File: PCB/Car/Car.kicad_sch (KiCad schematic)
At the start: 16 parts, among them J1 L1, J10 FL2, J11 FLT, J2 L2, J3 R1, J4 R2, J5 R1+2, J6 L1+2, J7 Conn_01x03, J8 pi zero 2 w, J9 FL1, U3 YAAJ_DCDC_StepDown_LM2596

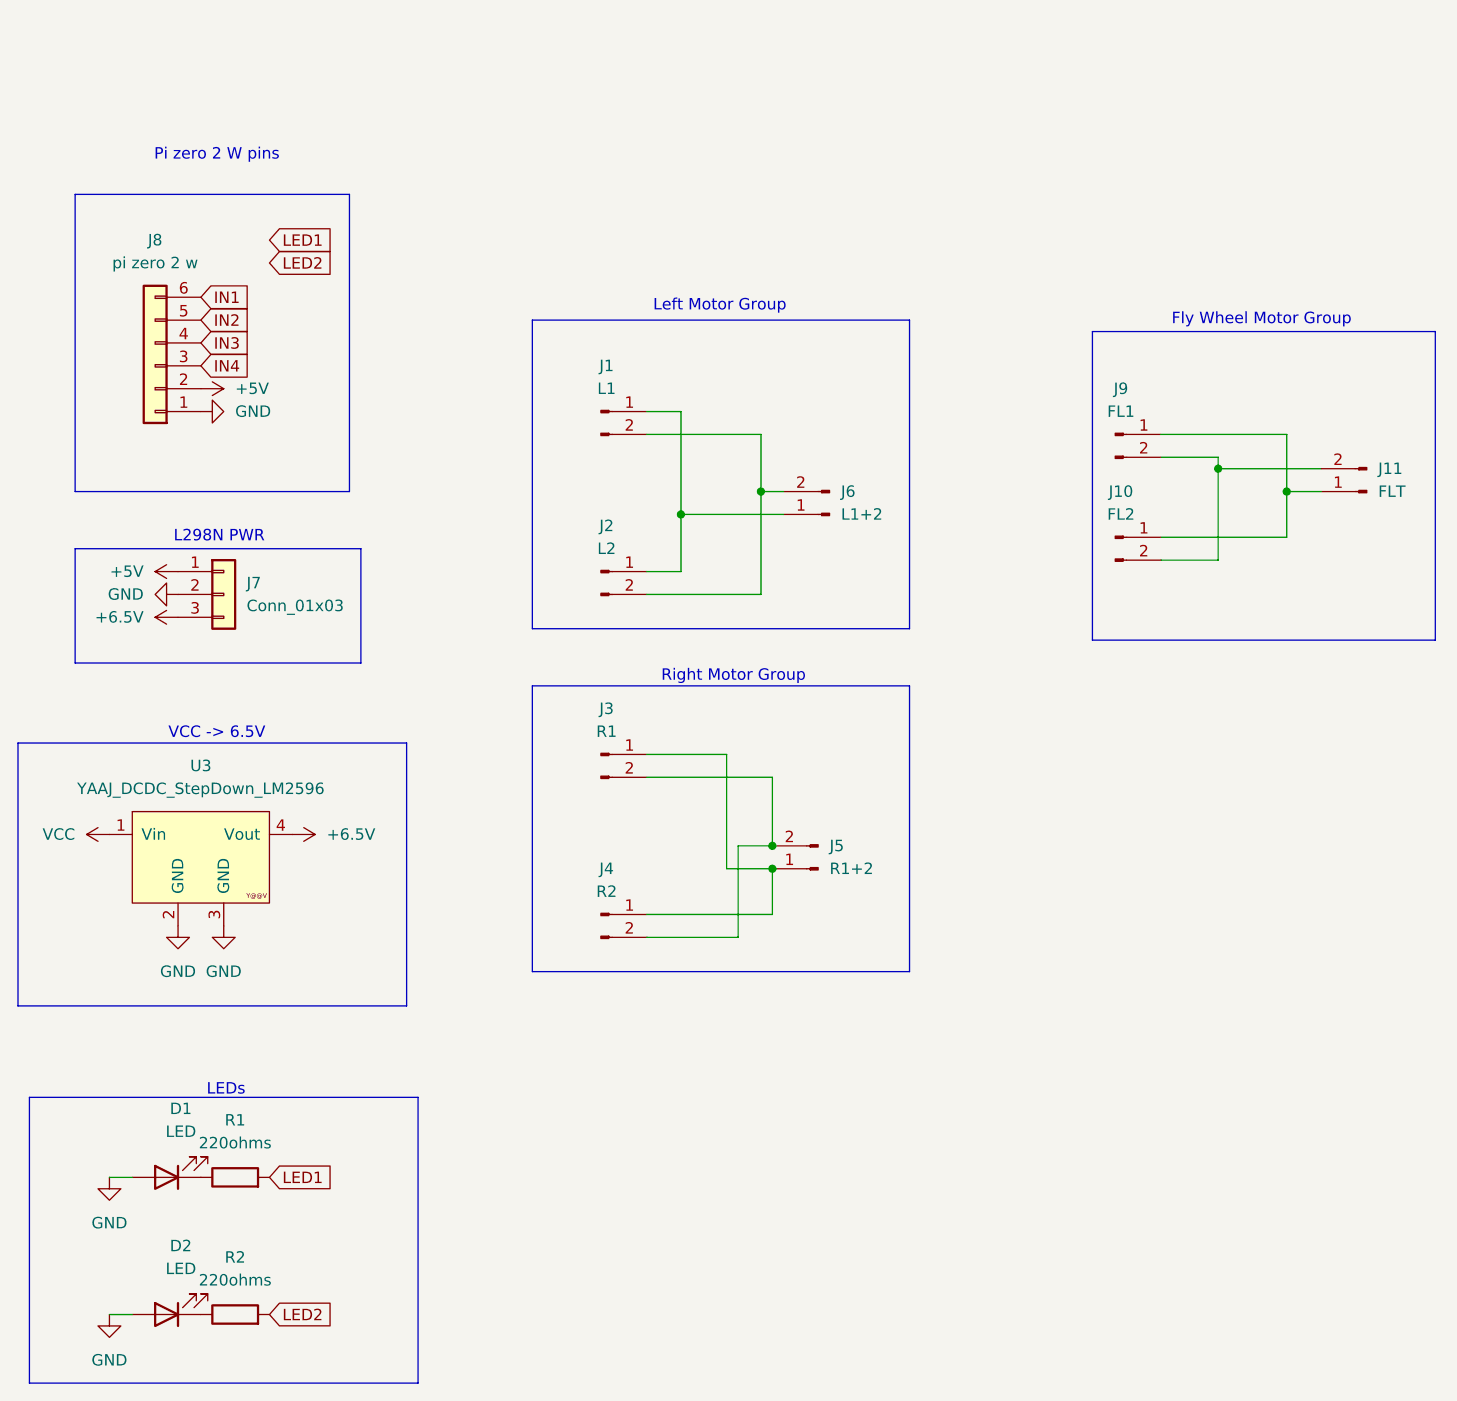
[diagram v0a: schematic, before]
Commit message: finish PCB
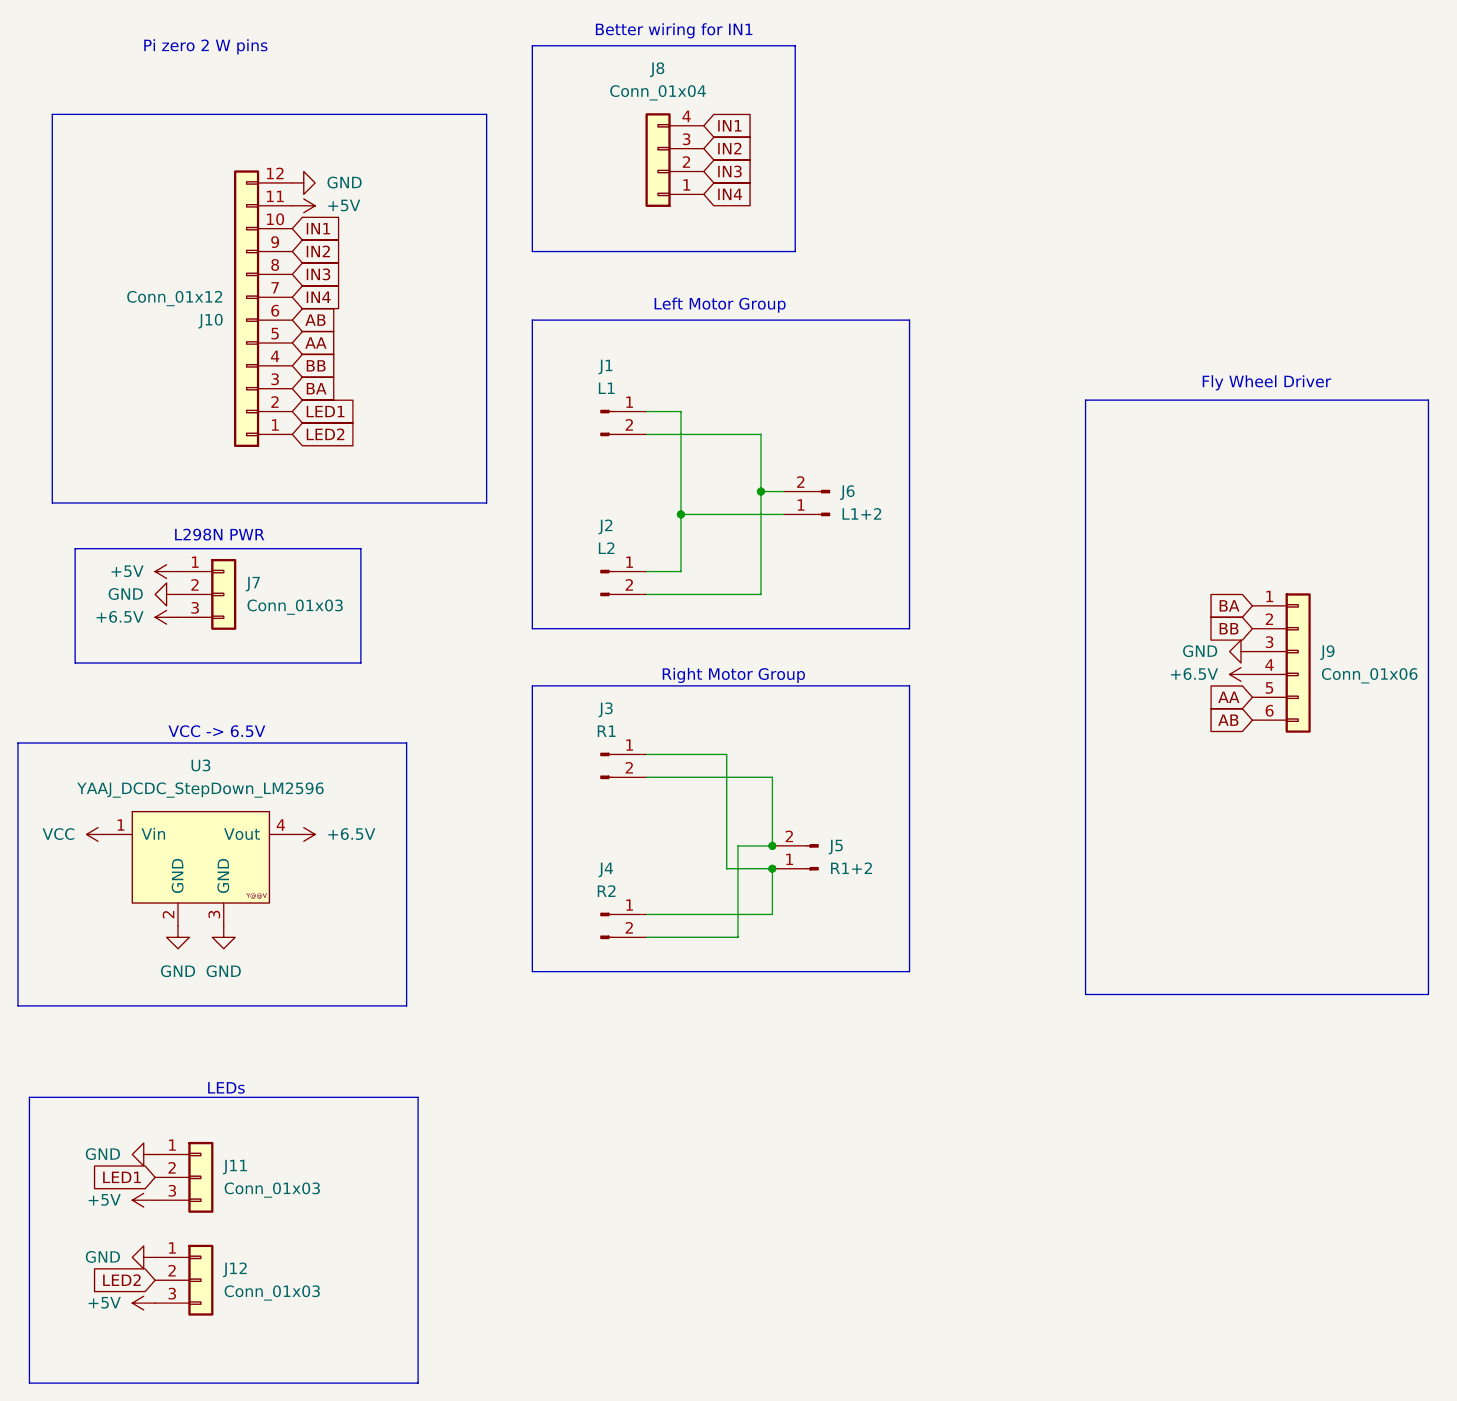
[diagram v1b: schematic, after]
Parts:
- removed D1, D2: LED, LED_THT:LED_D5.0mm, symbol Device:LED
- removed J10: FL2, Connector:JWT_A3963_1x02_P3.96mm_Vertical, symbol Connector:Conn_01x02_Pin
- removed J11: FLT, Connector:JWT_A3963_1x02_P3.96mm_Vertical, symbol Connector:Conn_01x02_Pin
- removed J8: pi zero 2 w, Connector_JST:JST_PH_B6B-PH-K_1x06_P2.00mm_Vertical, symbol Connector_Generic:Conn_01x06
- removed J9: FL1, Connector:JWT_A3963_1x02_P3.96mm_Vertical, symbol Connector:Conn_01x02_Pin
- removed R1, R2: 220ohms, Resistor_THT:R_Axial_DIN0207_L6.3mm_D2.5mm_P7.62mm_Horizontal, symbol Device:R
- added J10: Conn_01x12, Connector_PinHeader_2.54mm:PinHeader_1x12_P2.54mm_Vertical, symbol Connector_Generic:Conn_01x12
- added J11, J12: Conn_01x03, Connector:FanPinHeader_1x03_P2.54mm_Vertical, symbol Connector_Generic:Conn_01x03
- added J8: Conn_01x04, Connector:FanPinHeader_1x04_P2.54mm_Vertical, symbol Connector_Generic:Conn_01x04
- added J9: Conn_01x06, Connector_PinHeader_2.54mm:PinHeader_1x06_P2.54mm_Vertical, symbol Connector_Generic:Conn_01x06
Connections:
- net +5V: now also J10.11 (Pin_11), J11.3 (Pin_3), J12.3 (Pin_3)
- net +6.5V: now also J9.4 (Pin_4)
- net GND: now also J10.12 (Pin_12), J11.1 (Pin_1), J12.1 (Pin_1), J9.3 (Pin_3)
- net IN1: now also J10.10 (Pin_10), J8.4 (Pin_4)
- net IN2: now also J10.9 (Pin_9), J8.3 (Pin_3)
- net IN3: now also J10.8 (Pin_8), J8.2 (Pin_2)
- net IN4: now also J10.7 (Pin_7), J8.1 (Pin_1)
- net LED1: now also J10.2 (Pin_2), J11.2 (Pin_2)
- net LED2: now also J10.1 (Pin_1), J12.2 (Pin_2)
- new net AA: J10.5 (Pin_5), J9.5 (Pin_5)
- new net AB: J10.6 (Pin_6), J9.6 (Pin_6)
- new net BA: J10.3 (Pin_3), J9.1 (Pin_1)
- new net BB: J10.4 (Pin_4), J9.2 (Pin_2)
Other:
- note added: "Better wiring for IN1"
- note added: "Fly Wheel Driver"
- note removed: "Fly Wheel Motor Group"

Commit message: updated pcb :D
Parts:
- J1, J2, J3, J4, J5, J6: footprint Connector:JWT_A3963_1x02_P3.96mm_Vertical -> JST:JST 1x2
- J10: footprint Connector_PinHeader_2.54mm:PinHeader_1x12_P2.54mm_Vertical -> JST:JST 1x12
- J11, J12, J7: footprint Connector:FanPinHeader_1x03_P2.54mm_Vertical -> JST:JST 1x3
- J8: footprint Connector:FanPinHeader_1x04_P2.54mm_Vertical -> JST:JST 1x4
- J9: footprint Connector_PinHeader_2.54mm:PinHeader_1x06_P2.54mm_Vertical -> JST:JST 1x6
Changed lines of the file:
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@@
 			)
 		)
-		(property "Footprint" "Connector:FanPinHeader_1x03_P2.54mm_Vertical"
+		(property "Footprint" "JST:JST 1x3"
 			(at 57.15 102.87 0)
 			(effects
@@
 			)
 		)
-		(property "Footprint" "Connector:JWT_A3963_1x02_P3.96mm_Vertical"
+		(property "Footprint" "JST:JST 1x2"
 			(at 99.06 82.55 0)
 			(effects
@@
 			)
 		)
-		(property "Footprint" "Connector_PinHeader_2.54mm:PinHeader_1x12_P2.54mm_Vertical"
+		(property "Footprint" "JST:JST 1x12"
 			(at 59.69 72.39 0)
 			(effects
@@
 			)
 		)
-		(property "Footprint" "Connector:FanPinHeader_1x03_P2.54mm_Vertical"
+		(property "Footprint" "JST:JST 1x3"
 			(at 54.61 167.64 0)
 			(effects
@@
 			)
 		)
-		(property "Footprint" "Connector:JWT_A3963_1x02_P3.96mm_Vertical"
+		(property "Footprint" "JST:JST 1x2"
 			(at 123.19 133.35 0)
 			(effects
@@
 			)
 		)
-		(property "Footprint" "Connector_PinHeader_2.54mm:PinHeader_1x06_P2.54mm_Vertical"
+		(property "Footprint" "JST:JST 1x6"
 			(at 176.53 109.22 0)
 			(effects
@@
 			)
 		)
-		(property "Footprint" "Connector:JWT_A3963_1x02_P3.96mm_Vertical"
+		(property "Footprint" "JST:JST 1x2"
 			(at 99.06 100.33 0)
 			(effects
@@
 			)
 		)
-		(property "Footprint" "Connector:JWT_A3963_1x02_P3.96mm_Vertical"
+		(property "Footprint" "JST:JST 1x2"
 			(at 99.06 138.43 0)
 			(effects
@@
 			)
 		)
-		(property "Footprint" "Connector:JWT_A3963_1x02_P3.96mm_Vertical"
+		(property "Footprint" "JST:JST 1x2"
 			(at 99.06 120.65 0)
 			(effects
@@
 			)
 		)
-		(property "Footprint" "Connector:FanPinHeader_1x03_P2.54mm_Vertical"
+		(property "Footprint" "JST:JST 1x3"
 			(at 54.61 179.07 0)
 			(effects
@@
 			)
 		)
-		(property "Footprint" "Connector:FanPinHeader_1x04_P2.54mm_Vertical"
+		(property "Footprint" "JST:JST 1x4"
 			(at 105.41 55.88 0)
 			(effects
@@
 			)
 		)
-		(property "Footprint" "Connector:JWT_A3963_1x02_P3.96mm_Vertical"
+		(property "Footprint" "JST:JST 1x2"
 			(at 124.46 93.98 0)
 			(effects
